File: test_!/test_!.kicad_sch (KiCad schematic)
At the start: 25 parts, among them J1 Screw_Terminal_01x02, SW1 SW_Push, SW2 SW_Wuerth_450301014042, U1 LM2574N-5, U2 NE555P

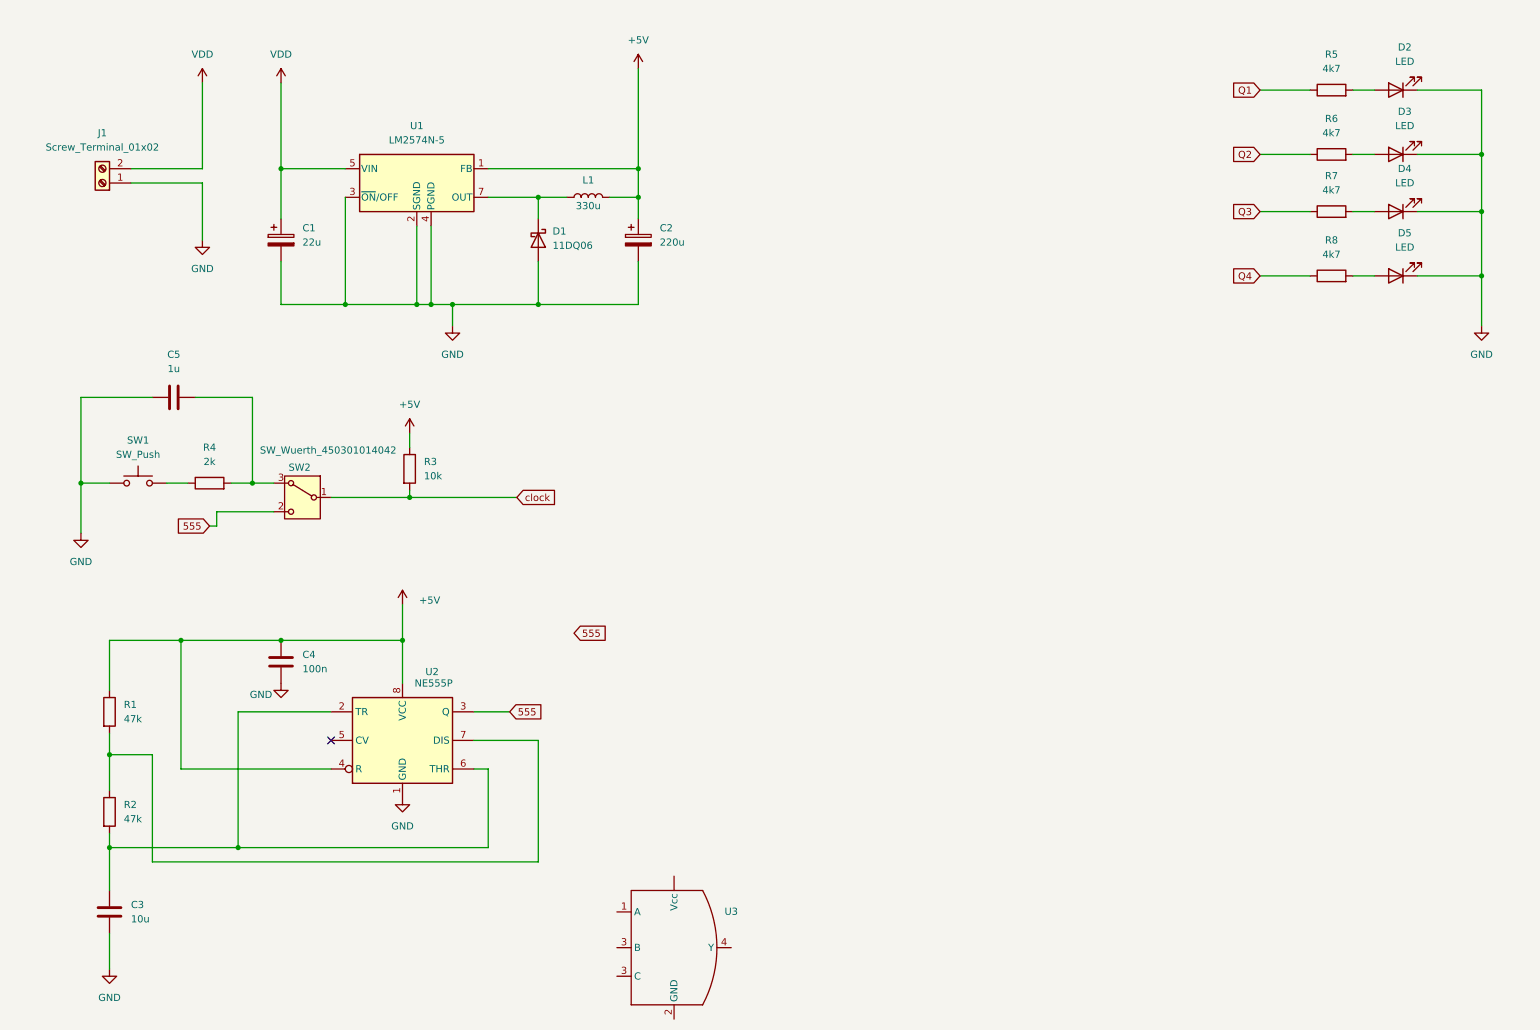
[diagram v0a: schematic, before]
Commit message: TEST
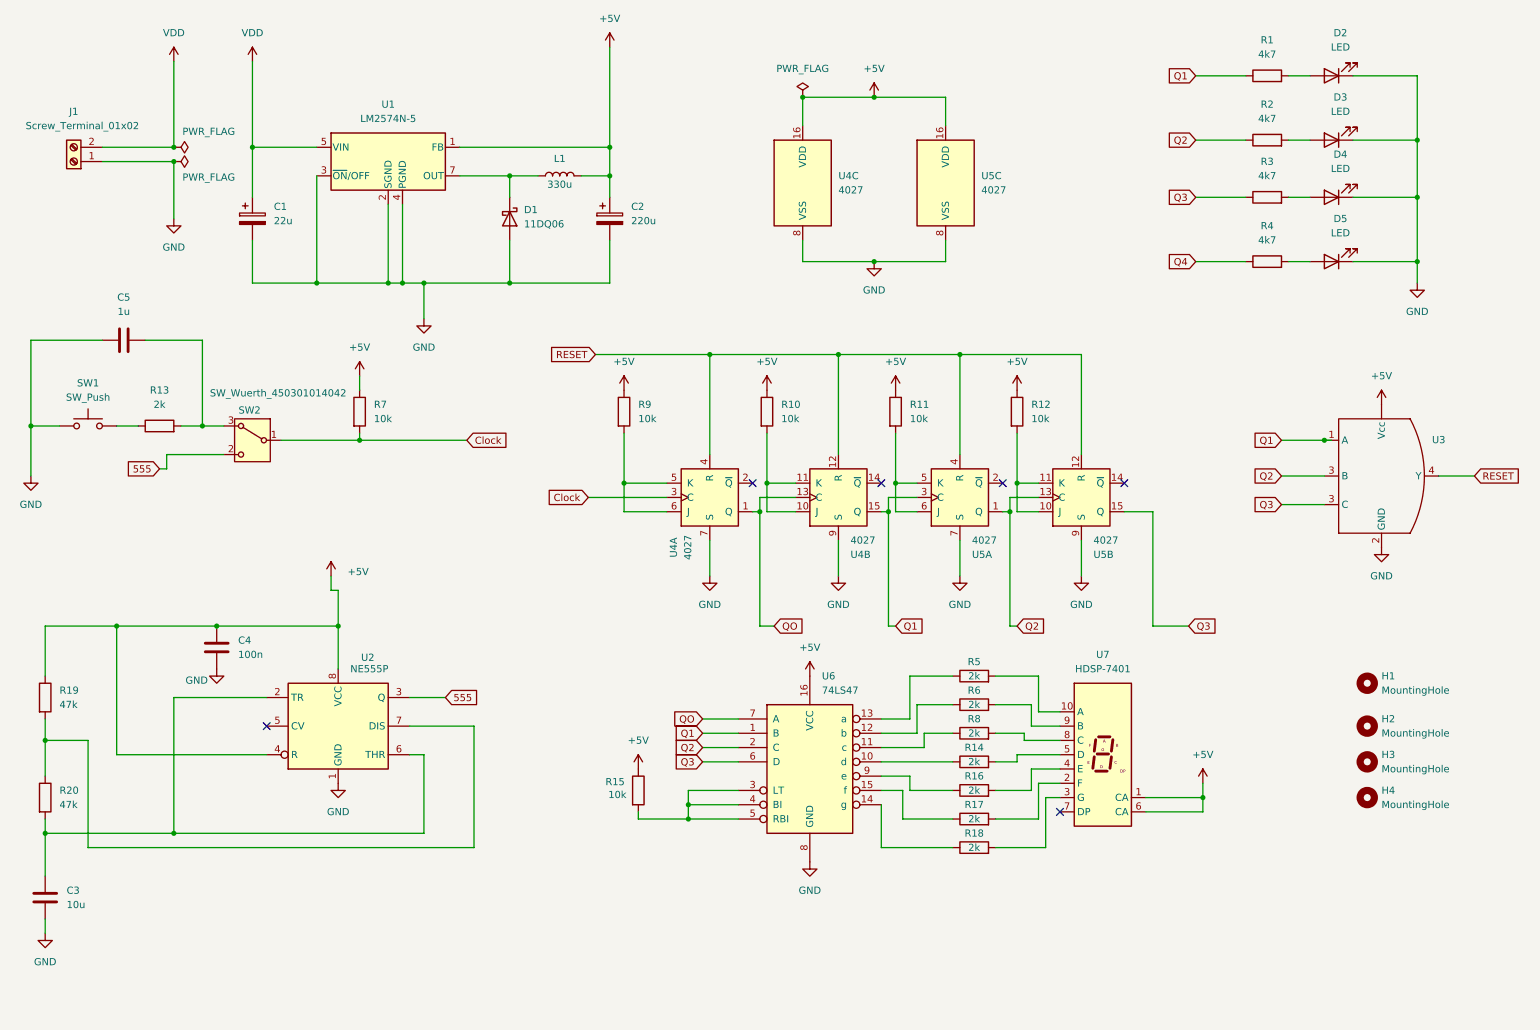
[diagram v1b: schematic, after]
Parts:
- added H1, H2, H3, H4: MountingHole, symbol Mechanical:MountingHole
- added R10, R11, R12, R15, R9: 10k, symbol Device:R
- added R14, R16, R17, R18, R5, R6, R8: 2k, symbol Device:R
- added U4, U5: 4027, symbol 4xxx:4027
- added U6: 74LS47, symbol 74xx:74LS47
- added U7: HDSP-7401, Display_7Segment:HDSP-7401, symbol Display_Character:HDSP-7401
- renumbered R5 to R1, R4 to R13, R1 to R19, R6 to R2, R2 to R20, R7 to R3, R8 to R4, R3 to R7
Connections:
- net +5V: now also U3. (Vcc), R10.1, R11.1, R12.1, R15.1, R9.1, U4.16 (VDD), U5.16 (VDD), U6.16 (VCC), U7.1 (CA), U7.6 (CA)
- net GND: now also U3.2 (GND), U4.7 (S), U4.8 (VSS), U4.9 (S), U5.7 (S), U5.8 (VSS), U5.9 (S), U6.8 (GND)
- net Q1: now also U3.1 (A), U4.15 (Q), U5.3 (C), U6.1 (B)
- net Q2: now also U3.3 (C), U5.1 (Q), U5.13 (C), U6.2 (C)
- net Q3: now also U3.3 (C), U5.15 (Q), U6.6 (D)
- net RESET: now reaches U3.4 (Y)
- net RESET: now also U4.12 (R), U4.4 (R), U5.12 (R), U5.4 (R)
- net clock renamed Clock
- net Clock: now also U4.3 (C)
- new net: R12.2, U5.10 (J), U5.11 (K)
- new net: R17.1, U6.15 (f)
- new net: R17.2, U7.2 (F)
- new net: R5.2, U7.10 (A)
- new net: R18.2, U7.3 (G)
- new net: R16.2, U7.4 (E)
- new net: R14.2, U7.5 (D)
- new net: R8.2, U7.8 (C)
- new net: R6.2, U7.9 (B)
- new net: R8.1, U6.11 (c)
- new net: R9.2, U4.5 (K), U4.6 (J)
- new net: R18.1, U6.14 (g)
- new net: R10.2, U4.10 (J), U4.11 (K)
- new net: R14.1, U6.10 (d)
- new net: R6.1, U6.12 (b)
- new net: R5.1, U6.13 (a)
- new net: R15.2, U6.3 (LT), U6.4 (BI), U6.5 (RBI)
- new net: R16.1, U6.9 (e)
- new net: R11.2, U5.5 (K), U5.6 (J)
- new net QO: U4.1 (Q), U4.13 (C), U6.7 (A)
- no-connect marks 1 -> 6
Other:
- title: (none) -> BCD Counter
- moved on the sheet: C1, C2, C3, C4, C5, D1, D2, D3, D4, D5, J1, L1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

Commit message: Doma
Domaca zadaca
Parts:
- C1, C2: footprint (none) -> Capacitor_THT:CP_Radial_D5.0mm_P2.00mm
- C3, C4, C5: footprint (none) -> Capacitor_SMD:C_1206_3216Metric_Pad1.33x1.80mm_HandSolder
- D1: footprint (none) -> Diode_THT:D_DO-41_SOD81_P10.16mm_Horizontal
- D2, D3, D4, D5: footprint (none) -> LED_THT:LED_D5.0mm
- H1, H2, H3, H4: footprint (none) -> MountingHole:MountingHole_5.5mm
- J1: footprint (none) -> TerminalBlock_MetzConnect:TerminalBlock_MetzConnect_Type011_RT05502HBLC_1x02_P5.00mm_Horizontal
- L1: footprint (none) -> Inductor_THT:L_Radial_D7.2mm_P3.00mm_Murata_1700
- R1, R2, R3, R4: footprint (none) -> Resistor_THT:R_Axial_DIN0207_L6.3mm_D2.5mm_P7.62mm_Horizontal
- R10, R11, R12, R13, R14, R15, R16, R17, R18, R19, R20, R5, R6, R7, R8, R9: footprint (none) -> Resistor_SMD:R_1206_3216Metric_Pad1.30x1.75mm_HandSolder
- SW1: footprint (none) -> Button_Switch_THT:SW_PUSH_6mm_H4.3mm
- U3, U4: footprint (none) -> Package_DIP:DIP-16_W7.62mm_Socket_LongPads
- U5: footprint (none) -> Display_7Segment:HDSP-7401
- U6: footprint (none) -> Package_TO_SOT_SMD:SOT-23-6
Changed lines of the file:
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@@
 			)
 		)
-		(property "Footprint" ""
+		(property "Footprint" "Display_7Segment:HDSP-7401"
 			(at 177.8 43.18 0)
 			(effects
@@
 			)
 		)
-		(property "Footprint" ""
+		(property "Footprint" "Display_7Segment:HDSP-7401"
 			(at 201.93 99.06 0)
 			(effects
@@
 			)
 		)
-		(property "Footprint" ""
+		(property "Footprint" "Resistor_SMD:R_1206_3216Metric_Pad1.30x1.75mm_HandSolder"
 			(at 182.88 157.988 90)
 			(effects
@@
 			)
 		)
-		(property "Footprint" ""
+		(property "Footprint" "Resistor_SMD:R_1206_3216Metric_Pad1.30x1.75mm_HandSolder"
 			(at 188.722 83.82 90)
 			(effects
@@
 			)
 		)
-		(property "Footprint" ""
+		(property "Footprint" "MountingHole:MountingHole_5.5mm"
 			(at 252.73 146.05 0)
 			(effects
@@
 			)
 		)
-		(property "Footprint" ""
+		(property "Footprint" "Resistor_SMD:R_1206_3216Metric_Pad1.30x1.75mm_HandSolder"
 			(at 71.882 83.82 90)
 			(effects
@@
 			)
 		)
-		(property "Footprint" ""
+		(property "Footprint" "Resistor_THT:R_Axial_DIN0207_L6.3mm_D2.5mm_P7.62mm_Horizontal"
 			(at 234.95 58.928 90)
 			(effects
@@
 			)
 		)
-		(property "Footprint" ""
+		(property "Footprint" "Resistor_SMD:R_1206_3216Metric_Pad1.30x1.75mm_HandSolder"
 			(at 16.002 134.62 90)
 			(effects
@@
 			)
 		)
-		(property "Footprint" ""
+		(property "Footprint" "Capacitor_THT:CP_Radial_D5.0mm_P2.00mm"
 			(at 119.0752 53.34 0)
 			(effects
@@
 			)
 		)
-		(property "Footprint" ""
+		(property "Footprint" "Resistor_SMD:R_1206_3216Metric_Pad1.30x1.75mm_HandSolder"
 			(at 182.88 142.748 90)
 			(effects
@@
 			)
 		)
-		(property "Footprint" ""
+		(property "Footprint" "Capacitor_SMD:C_1206_3216Metric_Pad1.33x1.80mm_HandSolder"
 			(at 49.2252 129.54 0)
 			(effects
@@
 			)
 		)
-		(property "Footprint" ""
+		(property "Footprint" "Diode_THT:D_DO-41_SOD81_P10.16mm_Horizontal"
 			(at 100.33 49.53 0)
 			(effects
@@
 			)
 		)
-		(property "Footprint" ""
+		(property "Footprint" "Resistor_SMD:R_1206_3216Metric_Pad1.30x1.75mm_HandSolder"
 			(at 118.872 83.82 90)
 			(effects
@@
 			)
 		)
-		(property "Footprint" ""
+		(property "Footprint" "Resistor_SMD:R_1206_3216Metric_Pad1.30x1.75mm_HandSolder"
 			(at 182.88 163.068 90)
 			(effects
@@
 			)
 		)
-		(property "Footprint" ""
+		(property "Footprint" "Resistor_THT:R_Axial_DIN0207_L6.3mm_D2.5mm_P7.62mm_Horizontal"
 			(at 234.95 47.498 90)
 			(effects
@@
 			)
 		)
-		(property "Footprint" ""
+		(property "Footprint" "Capacitor_SMD:C_1206_3216Metric_Pad1.33x1.80mm_HandSolder"
 			(at 18.7452 173.99 0)
 			(effects
@@
 			)
 		)
-		(property "Footprint" ""
+		(property "Footprint" "Button_Switch_THT:SW_PUSH_6mm_H4.3mm"
 			(at 25.4 81.28 0)
 			(effects
@@
 			)
 		)
-		(property "Footprint" ""
+		(property "Footprint" "Package_DIP:DIP-16_W7.62mm_Socket_LongPads"
 			(at 158.75 99.06 0)
 			(effects
@@
 			)
 		)
-		(property "Footprint" ""
+		(property "Footprint" "MountingHole:MountingHole_5.5mm"
 			(at 252.73 139.7 0)
 			(effects
@@
 			)
 		)
-		(property "Footprint" ""
+		(property "Footprint" "Package_TO_SOT_SMD:SOT-23-6"
 			(at 153.67 146.05 0)
 			(effects
@@
 			)
 		)
-		(property "Footprint" ""
+		(property "Footprint" "Display_7Segment:HDSP-7401"
 			(at 180.34 99.06 0)
 			(effects
@@
 			)
 		)
-		(property "Footprint" ""
+		(property "Footprint" "Package_DIP:DIP-16_W7.62mm_Socket_LongPads"
 			(at 135.89 99.06 0)
 			(effects
@@
 			)
 		)
-		(property "Footprint" ""
+		(property "Footprint" "Resistor_SMD:R_1206_3216Metric_Pad1.30x1.75mm_HandSolder"
 			(at 121.412 151.13 90)
 			(effects
@@
 			)
 		)
-		(property "Footprint" ""
+		(property "Footprint" "Resistor_THT:R_Axial_DIN0207_L6.3mm_D2.5mm_P7.62mm_Horizontal"
 			(at 234.95 25.908 90)
 			(effects
@@
 			)
 		)
-		(property "Footprint" ""
+		(property "Footprint" "LED_THT:LED_D5.0mm"
 			(at 246.38 35.56 0)
 			(effects
@@
 			)
 		)
-		(property "Footprint" ""
+		(property "Footprint" "Resistor_SMD:R_1206_3216Metric_Pad1.30x1.75mm_HandSolder"
 			(at 182.88 152.908 90)
 			(effects
@@
 			)
 		)
-		(property "Footprint" ""
+		(property "Footprint" "Resistor_SMD:R_1206_3216Metric_Pad1.30x1.75mm_HandSolder"
 			(at 182.88 132.588 90)
 			(effects
@@
 			)
 		)
-		(property "Footprint" ""
+		(property "Footprint" "Resistor_SMD:R_1206_3216Metric_Pad1.30x1.75mm_HandSolder"
 			(at 144.272 83.82 90)
 			(effects
@@
 			)
 		)
-		(property "Footprint" ""
+		(property "Footprint" "Resistor_SMD:R_1206_3216Metric_Pad1.30x1.75mm_HandSolder"
 			(at 167.132 83.82 90)
 			(effects
@@
 			)
 		)
-		(property "Footprint" ""
+		(property "Footprint" "MountingHole:MountingHole_5.5mm"
 			(at 252.73 132.08 0)
 			(effects
@@
 			)
 		)
-		(property "Footprint" ""
+		(property "Footprint" "LED_THT:LED_D5.0mm"
 			(at 246.38 57.15 0)
 			(effects
@@
 			)
 		)
-		(property "Footprint" ""
+		(property "Footprint" "TerminalBlock_MetzConnect:TerminalBlock_MetzConnect_Type011_RT05502HBLC_1x02_P5.00mm_Horizontal"
 			(at 22.86 39.37 0)
 			(effects
@@
 			)
 		)
-		(property "Footprint" ""
+		(property "Footprint" "Capacitor_SMD:C_1206_3216Metric_Pad1.33x1.80mm_HandSolder"
 			(at 27.94 72.0852 0)
 			(effects
@@
 			)
 		)
-		(property "Footprint" ""
+		(property "Footprint" "Capacitor_THT:CP_Radial_D5.0mm_P2.00mm"
 			(at 55.5752 53.34 0)
 			(effects
@@
 			)
 		)
-		(property "Footprint" ""
+		(property "Footprint" "Resistor_SMD:R_1206_3216Metric_Pad1.30x1.75mm_HandSolder"
 			(at 38.1 88.138 90)
 			(effects
@@
 			)
 		)
-		(property "Footprint" ""
+		(property "Footprint" "LED_THT:LED_D5.0mm"
 			(at 246.38 45.72 0)
 			(effects
@@
 			)
 		)
-		(property "Footprint" ""
+		(property "Footprint" "LED_THT:LED_D5.0mm"
 			(at 246.38 24.13 0)
 			(effects
@@
 			)
 		)
-		(property "Footprint" ""
+		(property "Footprint" "Inductor_THT:L_Radial_D7.2mm_P3.00mm_Murata_1700"
 			(at 109.22 41.91 0)
 			(effects
@@
 			)
 		)
-		(property "Footprint" ""
+		(property "Footprint" "Resistor_THT:R_Axial_DIN0207_L6.3mm_D2.5mm_P7.62mm_Horizontal"
 			(at 234.95 37.338 90)
 			(effects
@@
 			)
 		)
-		(property "Footprint" ""
+		(property "Footprint" "Package_DIP:DIP-16_W7.62mm_Socket_LongPads"
 			(at 247.65 81.28 0)
 			(effects
@@
 			)
 		)
-		(property "Footprint" ""
+		(property "Footprint" "Resistor_SMD:R_1206_3216Metric_Pad1.30x1.75mm_HandSolder"
 			(at 16.002 152.4 90)
 			(effects
@@
 			)
 		)
-		(property "Footprint" ""
+		(property "Footprint" "MountingHole:MountingHole_5.5mm"
 			(at 252.73 152.4 0)
 			(effects
@@
 			)
 		)
-		(property "Footprint" ""
+		(property "Footprint" "Resistor_SMD:R_1206_3216Metric_Pad1.30x1.75mm_HandSolder"
 			(at 182.88 137.668 90)
 			(effects
@@
 			)
 		)
-		(property "Footprint" ""
+		(property "Footprint" "Package_DIP:DIP-16_W7.62mm_Socket_LongPads"
 			(at 152.4 43.18 0)
 			(effects
@@
 			)
 		)
-		(property "Footprint" ""
+		(property "Footprint" "Resistor_SMD:R_1206_3216Metric_Pad1.30x1.75mm_HandSolder"
 			(at 182.88 147.828 90)
 			(effects
